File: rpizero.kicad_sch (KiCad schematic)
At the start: 1 part, among them U1 RASPBERRY_PI_ZERO_2_W

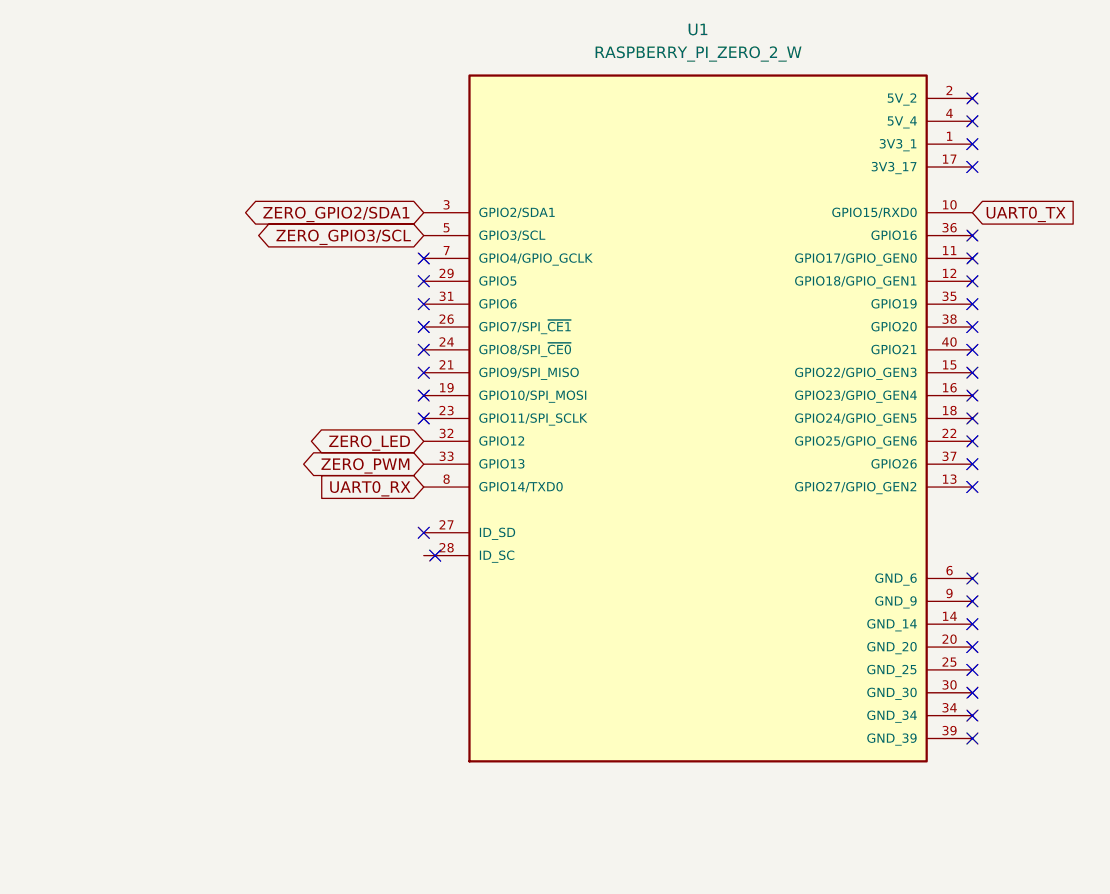
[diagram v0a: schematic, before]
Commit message: V1GD
V1 20/10/25
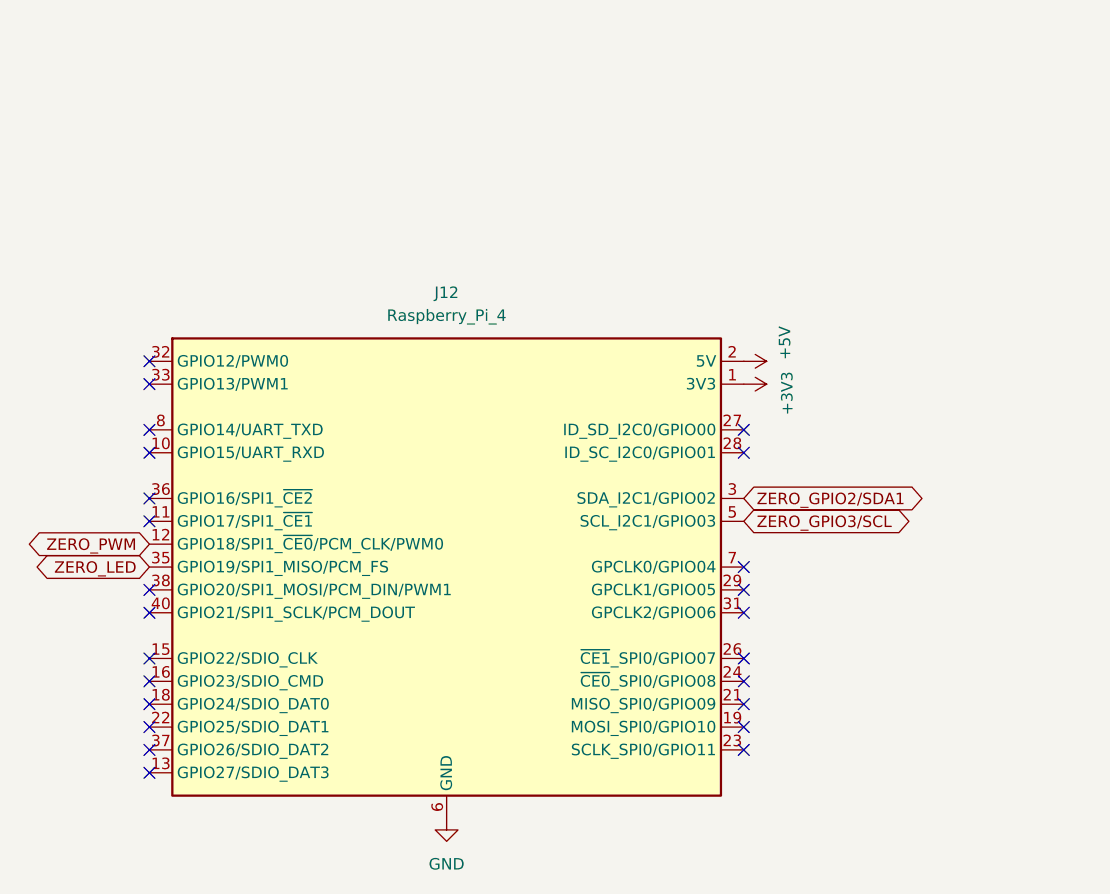
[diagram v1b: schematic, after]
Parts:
- removed U1: RASPBERRY_PI_ZERO_2_W, RASPBERRY_PI_ZERO_2_W:MODULE_RASPBERRY_PI_ZERO_2_W, symbol RASPBERRY_PI_ZERO_2_W:RASPBERRY_PI_ZERO_2_W
- added J12: Raspberry_Pi_4, symbol Connector:Raspberry_Pi_4
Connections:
- net ZERO_GPIO2/SDA1: now also J12.3 (SDA_I2C1/GPIO02)
- net ZERO_GPIO3/SCL: now also J12.5 (SCL_I2C1/GPIO03)
- net ZERO_LED: now also J12.35 (GPIO19/SPI1_MISO/PCM_FS)
- net ZERO_PWM: now also J12.12 (GPIO18/SPI1_~{CE0}/PCM_CLK/PWM0)
- new net +3V3: J12.1 (3V3), J12.17 (3V3)
- new net +5V: J12.2 (5V), J12.4 (5V)
- new net GND: J12.14 (GND), J12.20 (GND), J12.25 (GND), J12.30 (GND), J12.34 (GND), J12.39 (GND), J12.6 (GND), J12.9 (GND)
- no-connect marks 34 -> 24
